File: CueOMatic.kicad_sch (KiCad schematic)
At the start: 0 parts

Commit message: Initial pcb
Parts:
- added BT1: Battery_Cell, Connector_JST:JST_PH_B2B-PH-K_1x02_P2.00mm_Vertical, symbol Device:Battery_Cell
- added C1, C2: C_Polarized_Small, Capacitor_THT:CP_Radial_D5.0mm_P2.50mm, symbol Device:C_Polarized_Small
- added D1: WS2812B, LED_THT:LED_D5.0mm-4_RGB_Wide_Pins, symbol LED:WS2812B
- added J1: TTL, Connector_PinHeader_2.54mm:PinHeader_1x04_P2.54mm_Vertical, symbol Connector_Generic:Conn_01x04
- added J3: POGO_IN, Connector_PinHeader_2.54mm:PinHeader_1x05_P2.54mm_Vertical, symbol Connector_Generic:Conn_01x05
- added J4: POGO_OUT, Connector_PinHeader_2.54mm:PinHeader_1x05_P2.54mm_Vertical, symbol Connector_Generic:Conn_01x05
- added SW1: A, pts636:pts636, symbol Switch:SW_Push
- added SW2: MODE, pts636:pts636, symbol Switch:SW_Push
- added SW3: RESET, pts636:pts636, symbol Switch:SW_Push
- added SW4: SW_DIP_x04, Button_Switch_THT:SW_DIP_SPSTx04_Slide_6.7x11.72mm_W7.62mm_P2.54mm_LowProfile, symbol Switch:SW_DIP_x04
- added U1: ~, charge-module:charge-module, symbol charge-module:charge-module
- added U2: UA78M33_TO252, Package_TO_SOT_SMD:TO-252-2, symbol Regulator_Linear:KA78M05_TO252
- added U3: esp-01m, esp-01m:esp-01m, symbol esp-01m:esp-01m
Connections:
- new net: SW1.2, U3.7 (GP2)
- new net: BT1.1 (+), U1.4 (BAT+)
- new net: SW3.2, U3.18 (RST)
- new net: SW2.2, U3.8 (GP0)
- new net +3V3: C2.1, J1.4 (Pin_4), J3.2 (Pin_2), J4.2 (Pin_2), U2.3 (VO), U3.2 (VDD), U3.9 (EN)
- new net +5V: C1.1, D1.1 (VDD), U1.6 (VOUT), U2.1 (VI)
- new net DIP1: SW4.1, U3.14 (GP12)
- new net DIP2: SW4.2, U3.15 (GP14)
- new net DIP3: SW4.3, U3.16 (ADC)
- new net DIP4: SW4.4, U3.17 (GP16)
- new net GND: BT1.2 (-), C1.2, C2.2, D1.3 (VSS), J1.1 (Pin_1), J3.1 (Pin_1), J4.1 (Pin_1), SW1.1, SW2.1, SW3.1, SW4.5, SW4.6, SW4.7, SW4.8, U1.2 (GND), U1.3 (GND), U1.5 (GND), U2.2 (GND), U3.1 (GND)
- new net I2C_SCL: J3.4 (Pin_4), J4.4 (Pin_4), U3.13 (GP5)
- new net I2C_SDA: J3.3 (Pin_3), J4.3 (Pin_3), U3.12 (GP10)
- new net Neopixel: D1.4 (DIN), U3.11 (GP9)
- new net RX: J1.3 (Pin_3), U3.4 (GP3/RX)
- new net TX: J1.2 (Pin_2), U3.3 (GP2/TX)
- new net VBUS: J3.5 (Pin_5), J4.5 (Pin_5), U1.1 (VIN)
- no-connect marks 0 -> 1

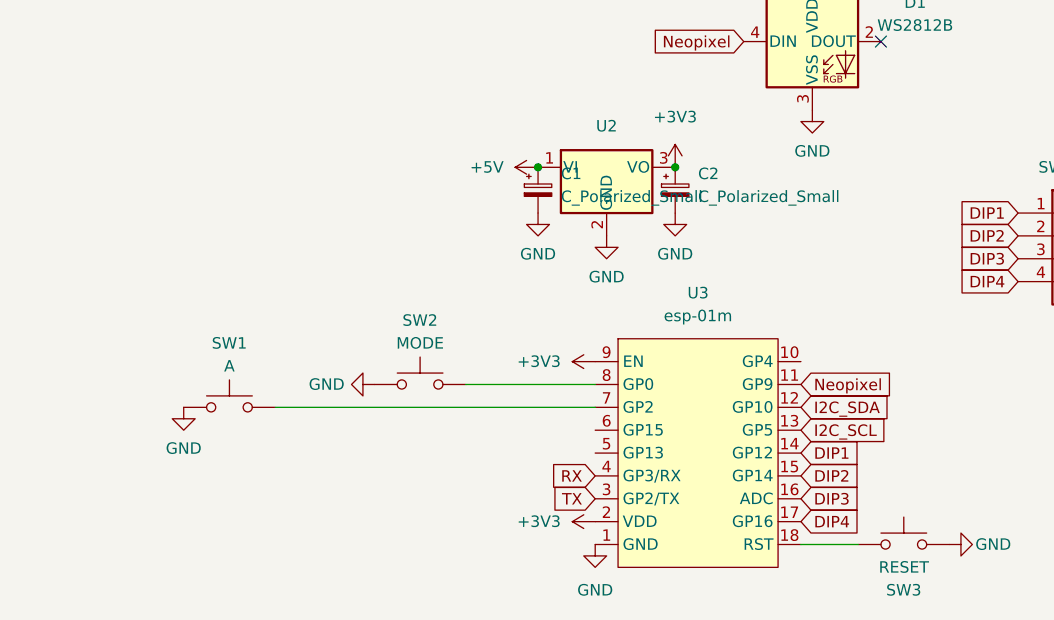
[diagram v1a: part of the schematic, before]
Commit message: Pre milling
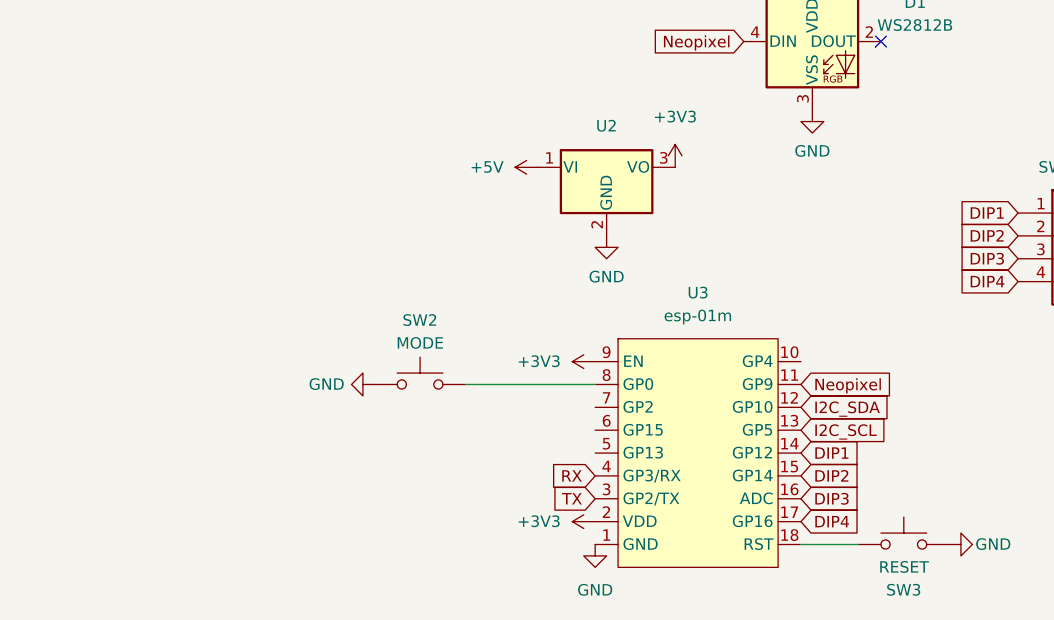
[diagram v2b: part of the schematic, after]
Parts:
- removed C1, C2: C_Polarized_Small, Capacitor_THT:CP_Radial_D5.0mm_P2.50mm, symbol Device:C_Polarized_Small
- removed SW1: A, pts636:pts636, symbol Switch:SW_Push
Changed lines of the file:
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@@
   (junction (at 232.41 121.92) (diameter 0) (color 0 0 0 0)
   )
-  (junction (at 179.07 109.22) (diameter 0) (color 0 0 0 0)
-  )
   (junction (at 232.41 116.84) (diameter 0) (color 0 0 0 0)
-  )
-  (junction (at 163.83 109.22) (diameter 0) (color 0 0 0 0)
   )
   (junction (at 232.41 119.38) (diameter 0) (color 0 0 0 0)
@@
   )
   (wire (pts (xy 193.04 151.13) (xy 199.39 151.13))
-    (stroke (width 0) (type default))
-  )
-  (wire (pts (xy 134.62 135.89) (xy 170.18 135.89))
     (stroke (width 0) (type default))
   )
@@
     )
   )
-  (symbol (lib_id "Switch:SW_Push") (at 129.54 135.89 0) (unit 1)
-    (in_bom yes) (on_board yes) (dnp no)
-    (property "Reference" "SW1" (at 129.54 128.778 0)
-      (effects (font (size 1.27 1.27)))
-    )
-    (property "Value" "A" (at 129.54 131.318 0)
-      (effects (font (size 1.27 1.27)))
-    )
-    (property "Footprint" "pts636:pts636" (at 129.54 130.81 0)
-      (effects (font (size 1.27 1.27)) hide)
-    )
-    (property "Datasheet" "~" (at 129.54 130.81 0)
-      (effects (font (size 1.27 1.27)) hide)
-    )
-    (pin "1")
-    (pin "2")
-    (instances
-      (project "CueOMatic"
-        (path "/10ca5df8-dddd-43fc-8084-86451cd2679c"
-          (reference "SW1") (unit 1)
-        )
-      )
-    )
-  )
   (symbol (lib_id "Regulator_Linear:KA78M05_TO252") (at 171.45 109.22 0) (unit 1)
     (in_bom yes) (on_board yes) (dnp no)
@@
         (path "/10ca5df8-dddd-43fc-8084-86451cd2679c"
           (reference "#PWR08") (unit 1)
-        )
-      )
-    )
-  )
-  (symbol (lib_id "Device:C_Polarized_Small") (at 179.07 111.76 0) (unit 1)
-    (in_bom yes) (on_board yes) (dnp no) (fields_autoplaced)
-    (property "Reference" "C2" (at 181.61 109.9438 0)
-      (effects (font (size 1.27 1.27)) (justify left))
-    )
-    (property "Value" "C_Polarized_Small" (at 181.61 112.4838 0)
-      (effects (font (size 1.27 1.27)) (justify left))
-    )
-    (property "Footprint" "Capacitor_THT:CP_Radial_D5.0mm_P2.50mm" (at 179.07 111.76 0)
-      (effects (font (size 1.27 1.27)) hide)
-    )
-    (property "Datasheet" "~" (at 179.07 111.76 0)
-      (effects (font (size 1.27 1.27)) hide)
-    )
-    (pin "1")
-    (pin "2")
-    (instances
-      (project "CueOMatic"
-        (path "/10ca5df8-dddd-43fc-8084-86451cd2679c"
-          (reference "C2") (unit 1)
         )
       )
@@
     )
   )
-  (symbol (lib_id "power:GND") (at 124.46 135.89 0) (unit 1)
-    (in_bom yes) (on_board yes) (dnp no) (fields_autoplaced)
-    (property "Reference" "#PWR01" (at 124.46 142.24 0)
-      (effects (font (size 1.27 1.27)) hide)
-    )
-    (property "Value" "GND" (at 124.46 140.462 0)
-      (effects (font (size 1.27 1.27)))
-    )
-    (property "Footprint" "" (at 124.46 135.89 0)
-      (effects (font (size 1.27 1.27)) hide)
-    )
-    (property "Datasheet" "" (at 124.46 135.89 0)
-      (effects (font (size 1.27 1.27)) hide)
-    )
-    (pin "1")
-    (instances
-      (project "CueOMatic"
-        (path "/10ca5df8-dddd-43fc-8084-86451cd2679c"
-          (reference "#PWR01") (unit 1)
-        )
-      )
-    )
-  )
   (symbol (lib_id "power:GND") (at 121.92 81.28 0) (unit 1)
     (in_bom yes) (on_board yes) (dnp no) (fields_autoplaced)
@@
     )
   )
-  (symbol (lib_id "power:GND") (at 179.07 114.3 0) (unit 1)
-    (in_bom yes) (on_board yes) (dnp no) (fields_autoplaced)
-    (property "Reference" "#PWR010" (at 179.07 120.65 0)
-      (effects (font (size 1.27 1.27)) hide)
-    )
-    (property "Value" "GND" (at 179.07 118.872 0)
-      (effects (font (size 1.27 1.27)))
-    )
-    (property "Footprint" "" (at 179.07 114.3 0)
-      (effects (font (size 1.27 1.27)) hide)
-    )
-    (property "Datasheet" "" (at 179.07 114.3 0)
-      (effects (font (size 1.27 1.27)) hide)
-    )
-    (pin "1")
-    (instances
-      (project "CueOMatic"
-        (path "/10ca5df8-dddd-43fc-8084-86451cd2679c"
-          (reference "#PWR010") (unit 1)
-        )
-      )
-    )
-  )
-  (symbol (lib_id "Device:C_Polarized_Small") (at 163.83 111.76 0) (unit 1)
-    (in_bom yes) (on_board yes) (dnp no) (fields_autoplaced)
-    (property "Reference" "C1" (at 166.37 109.9438 0)
-      (effects (font (size 1.27 1.27)) (justify left))
-    )
-    (property "Value" "C_Polarized_Small" (at 166.37 112.4838 0)
-      (effects (font (size 1.27 1.27)) (justify left))
-    )
-    (property "Footprint" "Capacitor_THT:CP_Radial_D5.0mm_P2.50mm" (at 163.83 111.76 0)
-      (effects (font (size 1.27 1.27)) hide)
-    )
-    (property "Datasheet" "~" (at 163.83 111.76 0)
-      (effects (font (size 1.27 1.27)) hide)
-    )
-    (pin "1")
-    (pin "2")
-    (instances
-      (project "CueOMatic"
-        (path "/10ca5df8-dddd-43fc-8084-86451cd2679c"
-          (reference "C1") (unit 1)
-        )
-      )
-    )
-  )
   (symbol (lib_id "Switch:SW_Push") (at 204.47 151.13 0) (mirror y) (unit 1)
     (in_bom yes) (on_board yes) (dnp no)
@@
         )
       )
-    )
-  )
-  (symbol (lib_id "power:GND") (at 163.83 114.3 0) (unit 1)
-    (in_bom yes) (on_board yes) (dnp no) (fields_autoplaced)
-    (property "Reference" "#PWR04" (at 163.83 120.65 0)
-      (effects (font (size 1.27 1.27)) hide)
-    )
-    (property "Value" "GND" (at 163.83 118.872 0)
-      (effects (font (size 1.27 1.27)))
-    )
-    (property "Footprint" "" (at 163.83 114.3 0)
-      (effects (font (size 1.27 1.27)) hide)
-    )
-    (property "Datasheet" "" (at 163.83 114.3 0)
-      (effects (font (size 1.27 1.27)) hide)
-    )
-    (pin "1")
-    (instances
-      (project "CueOMatic"
-        (path "/10ca5df8-dddd-43fc-8084-86451cd2679c"
-          (reference "#PWR04") (unit 1)
-        )
-      )

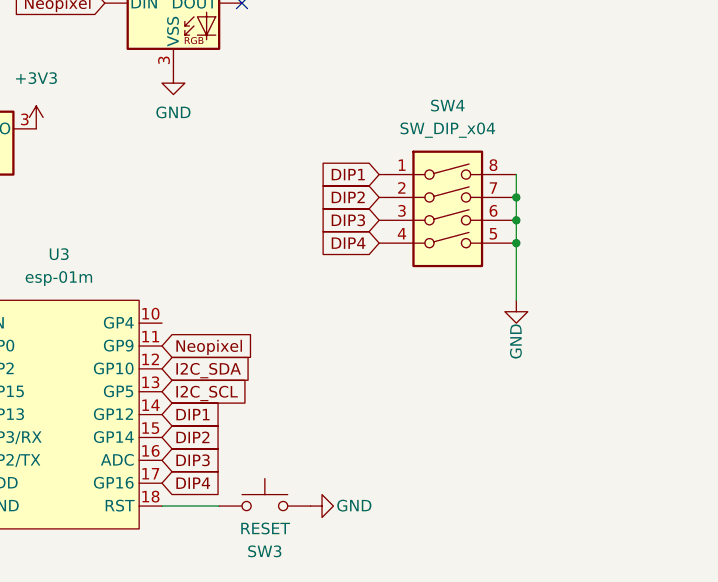
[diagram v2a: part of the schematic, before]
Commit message: Schematic remarks
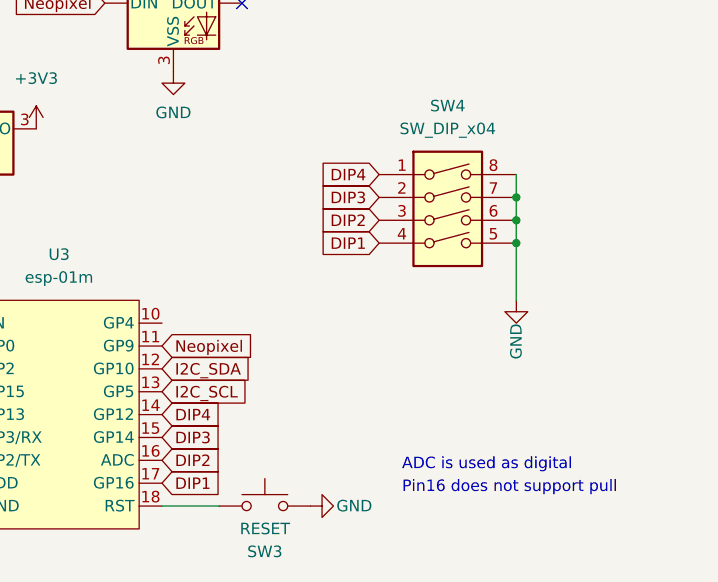
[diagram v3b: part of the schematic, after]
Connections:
- net DIP1: now also SW4.4, U3.17 (GP16); no longer SW4.1, U3.14 (GP12)
- net DIP2: now also SW4.3, U3.16 (ADC); no longer SW4.2, U3.15 (GP14)
- net DIP3: now also SW4.2, U3.15 (GP14); no longer SW4.3, U3.16 (ADC)
- net DIP4: now also SW4.1, U3.14 (GP12); no longer SW4.4, U3.17 (GP16)
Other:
- note added: "ADC is used as digital"
- note added: "Pin16 does not support pull"
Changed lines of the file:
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@@
     (stroke (width 0) (type default))
+  )
+  (text "ADC is used as digital" (at 219.71 147.32 0)
+    (effects (font (size 1.27 1.27)) (justify left bottom))
+  )
+  (text "Pin16 does not support pull" (at 219.71 149.86 0)
+    (effects (font (size 1.27 1.27)) (justify left bottom))
   )
   (global_label "I2C_SDA" (shape input) (at 232.41 54.61 0) (fields_autoplaced)
@@
     )
   )
-  (global_label "DIP1" (shape input) (at 193.04 140.97 0) (fields_autoplaced)
+  (global_label "DIP1" (shape input) (at 193.04 148.59 0) (fields_autoplaced)
     (effects (font (size 1.27 1.27)) (justify left))
-    (property "Intersheetrefs" "${INTERSHEET_REFS}" (at 200.3795 140.97 0)
+    (property "Intersheetrefs" "${INTERSHEET_REFS}" (at 200.3795 148.59 0)
       (effects (font (size 1.27 1.27)) (justify left) hide)
     )
@@
     )
   )
-  (global_label "DIP3" (shape input) (at 193.04 146.05 0) (fields_autoplaced)
+  (global_label "DIP3" (shape input) (at 193.04 143.51 0) (fields_autoplaced)
     (effects (font (size 1.27 1.27)) (justify left))
-    (property "Intersheetrefs" "${INTERSHEET_REFS}" (at 200.3795 146.05 0)
+    (property "Intersheetrefs" "${INTERSHEET_REFS}" (at 200.3795 143.51 0)
       (effects (font (size 1.27 1.27)) (justify left) hide)
     )
@@
     )
   )
-  (global_label "DIP4" (shape input) (at 193.04 148.59 0) (fields_autoplaced)
+  (global_label "DIP4" (shape input) (at 193.04 140.97 0) (fields_autoplaced)
     (effects (font (size 1.27 1.27)) (justify left))
-    (property "Intersheetrefs" "${INTERSHEET_REFS}" (at 200.3795 148.59 0)
+    (property "Intersheetrefs" "${INTERSHEET_REFS}" (at 200.3795 140.97 0)
       (effects (font (size 1.27 1.27)) (justify left) hide)
     )
   )
-  (global_label "DIP1" (shape input) (at 217.17 114.3 180) (fields_autoplaced)
+  (global_label "DIP1" (shape input) (at 217.17 121.92 180) (fields_autoplaced)
     (effects (font (size 1.27 1.27)) (justify right))
-    (property "Intersheetrefs" "${INTERSHEET_REFS}" (at 209.8305 114.3 0)
+    (property "Intersheetrefs" "${INTERSHEET_REFS}" (at 209.8305 121.92 0)
       (effects (font (size 1.27 1.27)) (justify right) hide)
     )
@@
     )
   )
-  (global_label "DIP2" (shape input) (at 193.04 143.51 0) (fields_autoplaced)
+  (global_label "DIP2" (shape input) (at 193.04 146.05 0) (fields_autoplaced)
     (effects (font (size 1.27 1.27)) (justify left))
-    (property "Intersheetrefs" "${INTERSHEET_REFS}" (at 200.3795 143.51 0)
+    (property "Intersheetrefs" "${INTERSHEET_REFS}" (at 200.3795 146.05 0)
       (effects (font (size 1.27 1.27)) (justify left) hide)
     )
@@
     )
   )
-  (global_label "DIP3" (shape input) (at 217.17 119.38 180) (fields_autoplaced)
+  (global_label "DIP3" (shape input) (at 217.17 116.84 180) (fields_autoplaced)
     (effects (font (size 1.27 1.27)) (justify right))
-    (property "Intersheetrefs" "${INTERSHEET_REFS}" (at 209.8305 119.38 0)
+    (property "Intersheetrefs" "${INTERSHEET_REFS}" (at 209.8305 116.84 0)
       (effects (font (size 1.27 1.27)) (justify right) hide)
     )
   )
-  (global_label "DIP4" (shape input) (at 217.17 121.92 180) (fields_autoplaced)
+  (global_label "DIP4" (shape input) (at 217.17 114.3 180) (fields_autoplaced)
     (effects (font (size 1.27 1.27)) (justify right))
-    (property "Intersheetrefs" "${INTERSHEET_REFS}" (at 209.8305 121.92 0)
+    (property "Intersheetrefs" "${INTERSHEET_REFS}" (at 209.8305 114.3 0)
       (effects (font (size 1.27 1.27)) (justify right) hide)
     )
@@
     )
   )
-  (global_label "DIP2" (shape input) (at 217.17 116.84 180) (fields_autoplaced)
+  (global_label "DIP2" (shape input) (at 217.17 119.38 180) (fields_autoplaced)
     (effects (font (size 1.27 1.27)) (justify right))
-    (property "Intersheetrefs" "${INTERSHEET_REFS}" (at 209.8305 116.84 0)
+    (property "Intersheetrefs" "${INTERSHEET_REFS}" (at 209.8305 119.38 0)
       (effects (font (size 1.27 1.27)) (justify right) hide)
     )
